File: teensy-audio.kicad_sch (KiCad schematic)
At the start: 44 parts, among them J1 AudioJack2, J2 AudioJack2, J3 Barrel_Jack, J4 Conn_02x08_Odd_Even, J5 Conn_02x08_Odd_Even, J6 Conn_02x05_Odd_Even, J7 Conn_01x04, SW1 RotaryEncoder_Switch, SW2 SW_Push, SW3 SW_Push, SW4 SW_Push, SW5 SW_Push, U1 LM358, U2 LM7805_TO220, U3 Teensy4.0, U4 Teensy4.0_AudioShield_REVD

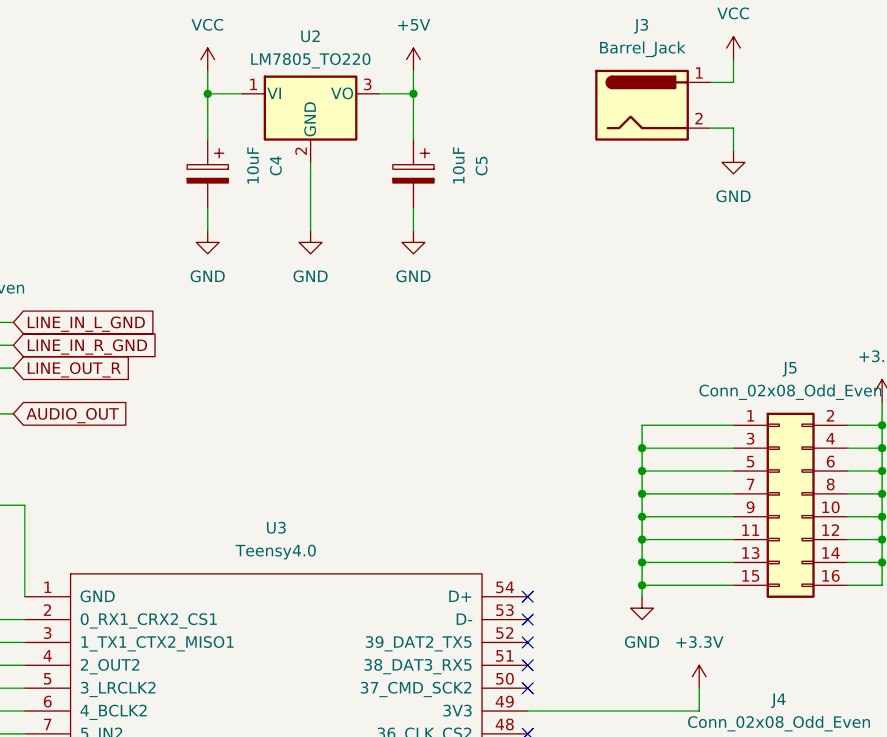
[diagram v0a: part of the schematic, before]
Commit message: added power connectors
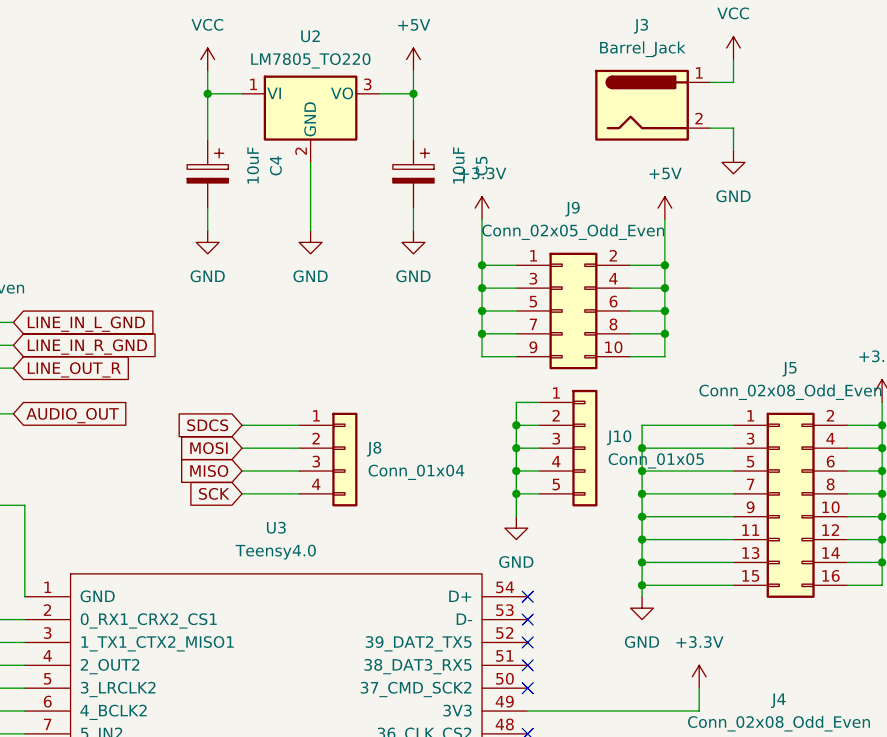
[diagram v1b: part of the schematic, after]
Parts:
- added J10: Conn_01x05, Connector_PinHeader_2.54mm:PinHeader_1x05_P2.54mm_Vertical, symbol Connector_Generic:Conn_01x05
- added J8: Conn_01x04, Connector_PinHeader_2.54mm:PinHeader_1x04_P2.54mm_Vertical, symbol Connector_Generic:Conn_01x04
- added J9: Conn_02x05_Odd_Even, Connector_PinHeader_2.54mm:PinHeader_2x05_P2.54mm_Vertical, symbol Connector_Generic:Conn_02x05_Odd_Even
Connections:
- net +3.3V: now also J9.1 (Pin_1), J9.3 (Pin_3), J9.5 (Pin_5), J9.7 (Pin_7), J9.9 (Pin_9)
- net +5V: now also J9.10 (Pin_10), J9.2 (Pin_2), J9.4 (Pin_4), J9.6 (Pin_6), J9.8 (Pin_8)
- net GND: now also J10.1 (Pin_1), J10.2 (Pin_2), J10.3 (Pin_3), J10.4 (Pin_4), J10.5 (Pin_5)
- net MISO: now also J8.3 (Pin_3)
- net MOSI: now also J8.2 (Pin_2)
- net SCK: now also J8.4 (Pin_4)
- net SDCS: now also J8.1 (Pin_1)
